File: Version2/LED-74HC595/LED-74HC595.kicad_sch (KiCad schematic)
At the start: 5 parts, among them J1 Conn_01x08_Pin, J2 Conn_01x08_Pin, J3 Conn_02x08_Odd_Even, U2 74HC595, U3 74HC595

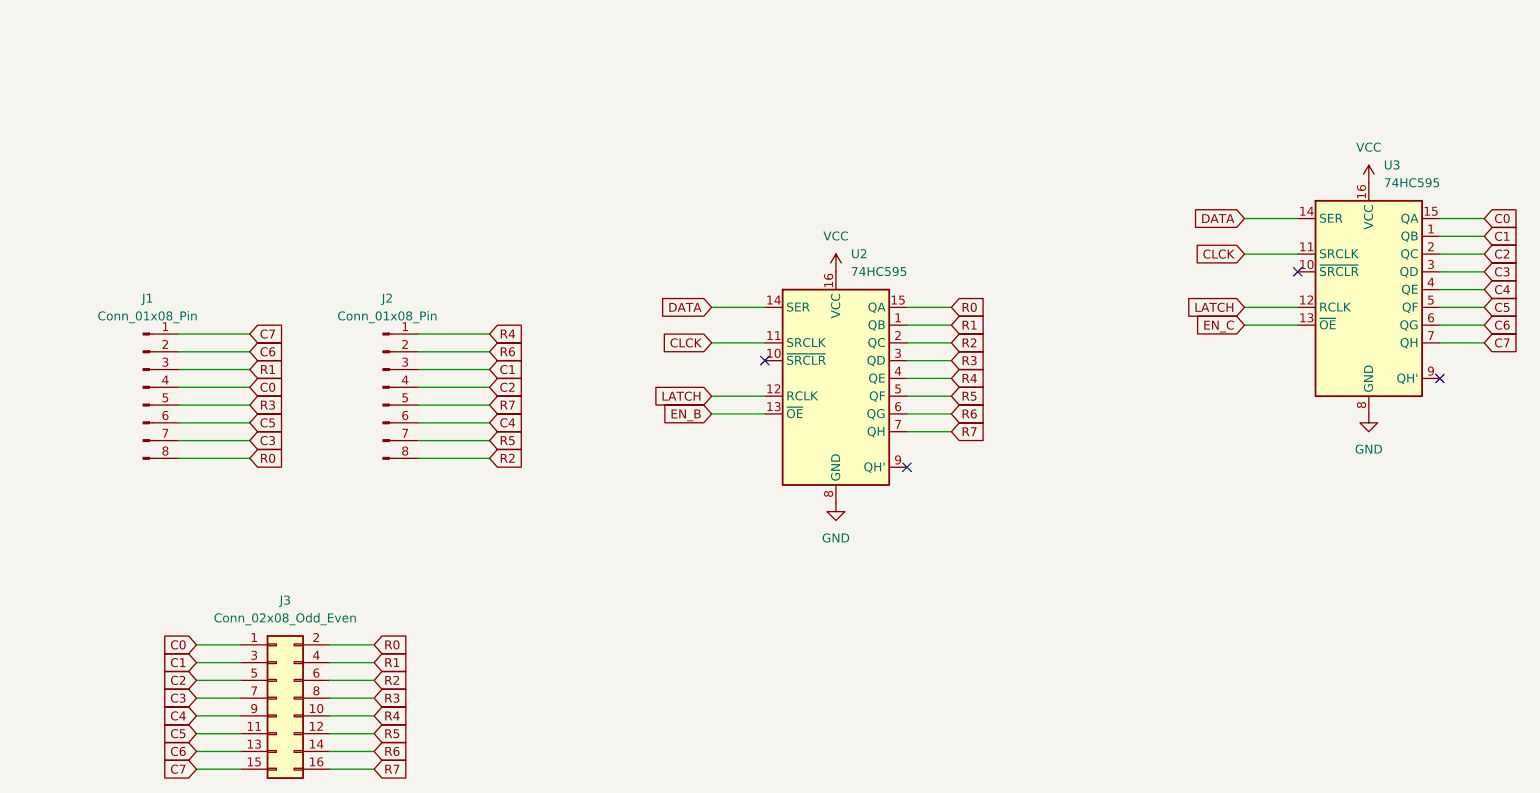
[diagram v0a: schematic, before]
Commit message: did some works.
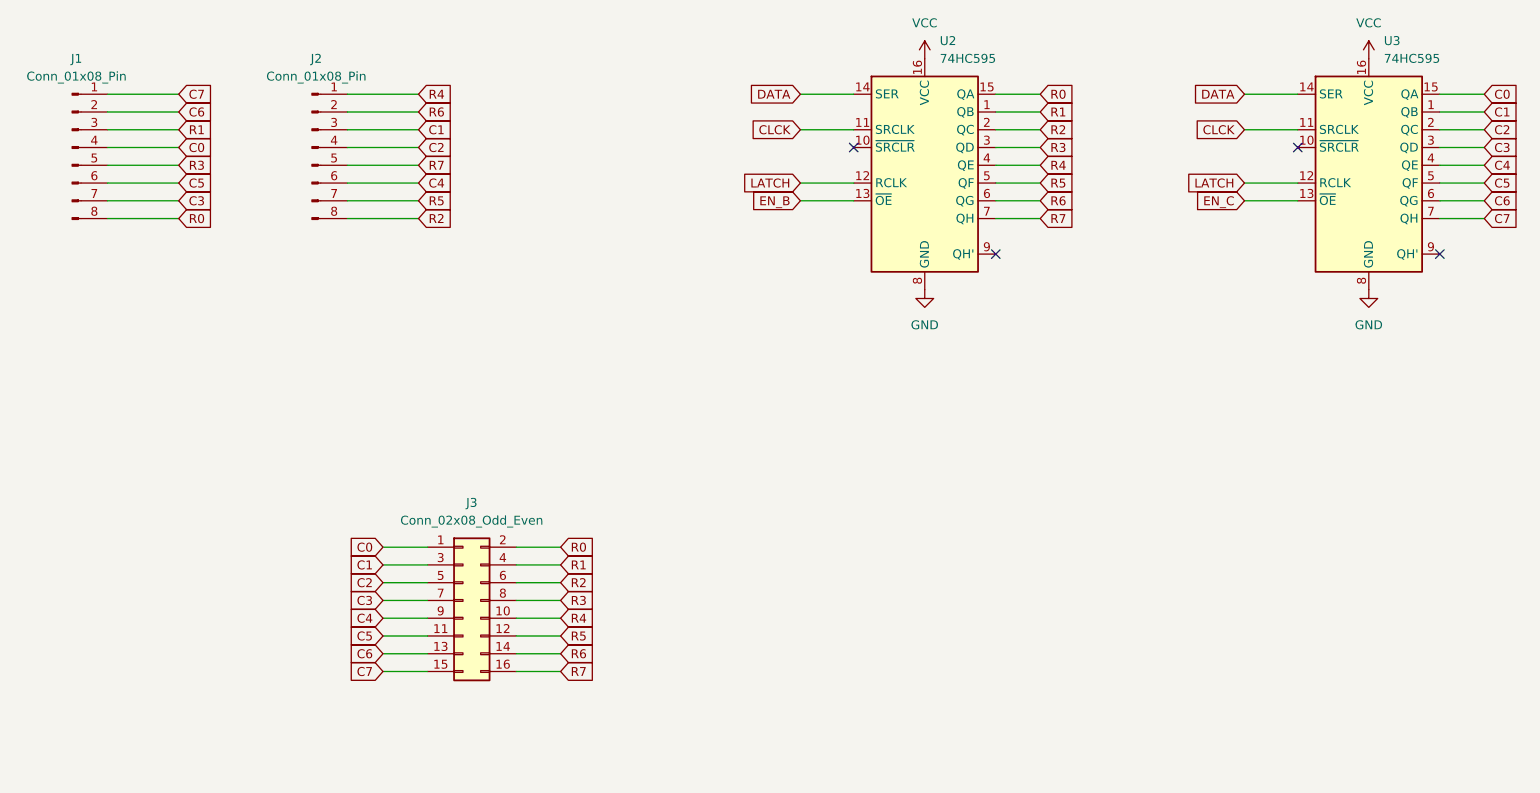
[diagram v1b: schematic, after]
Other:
- moved on the sheet: J1, J2, J3, U2, U3

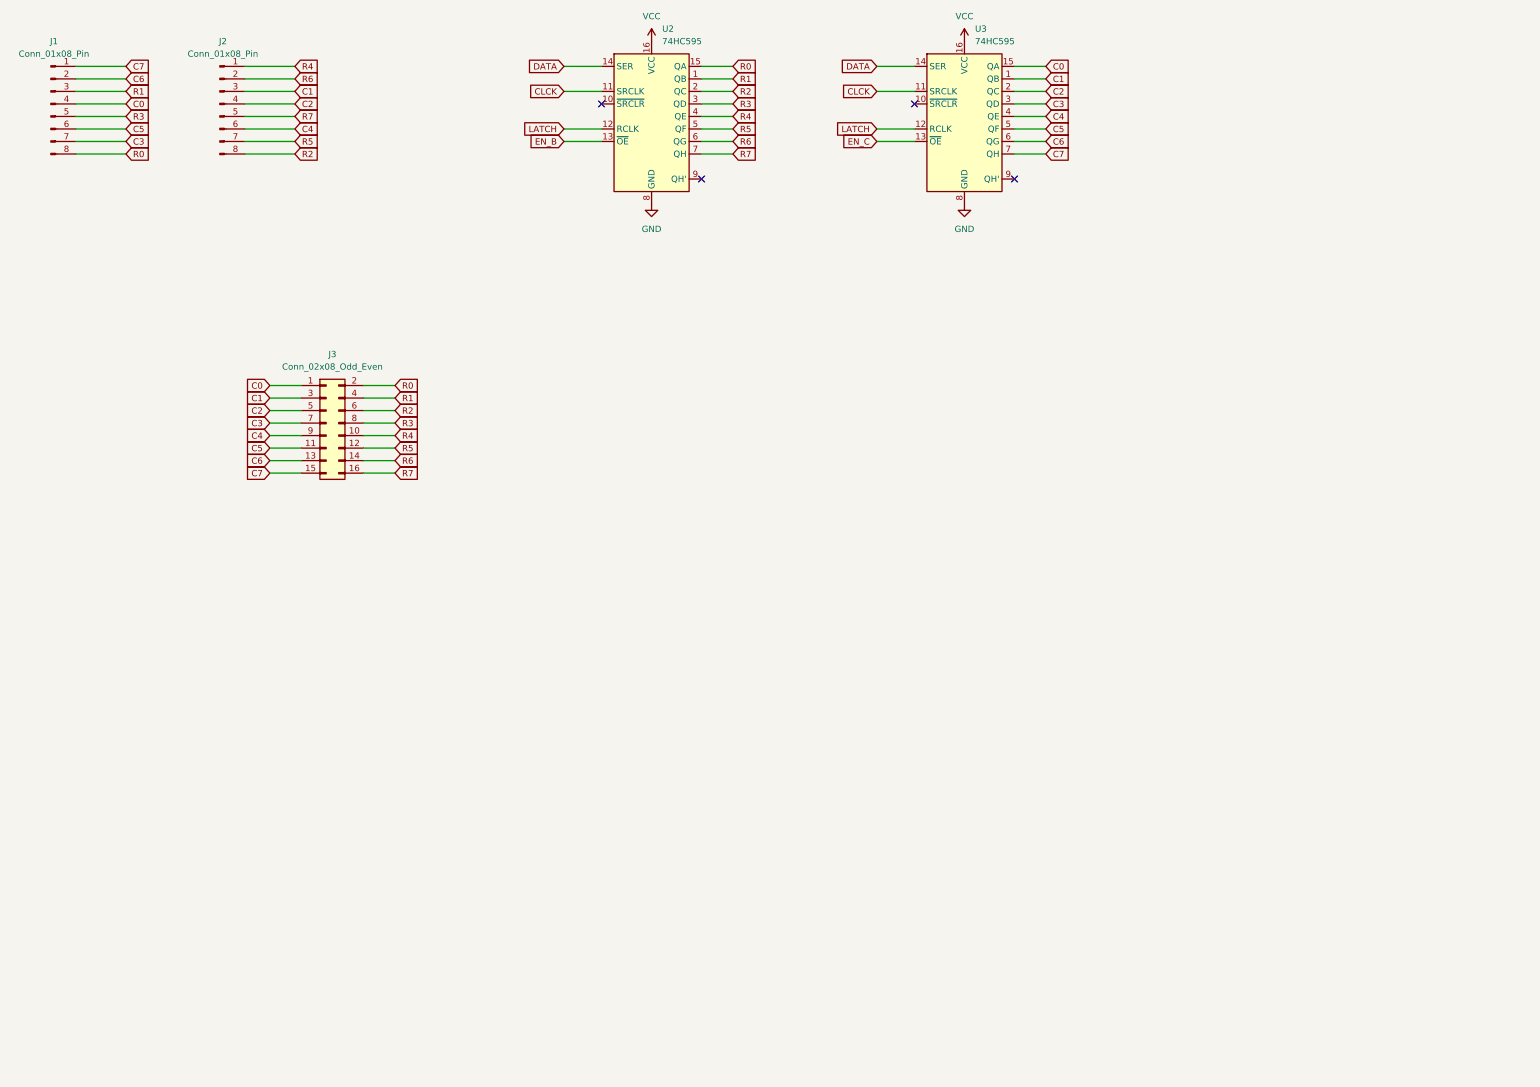
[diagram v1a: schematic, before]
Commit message: update.
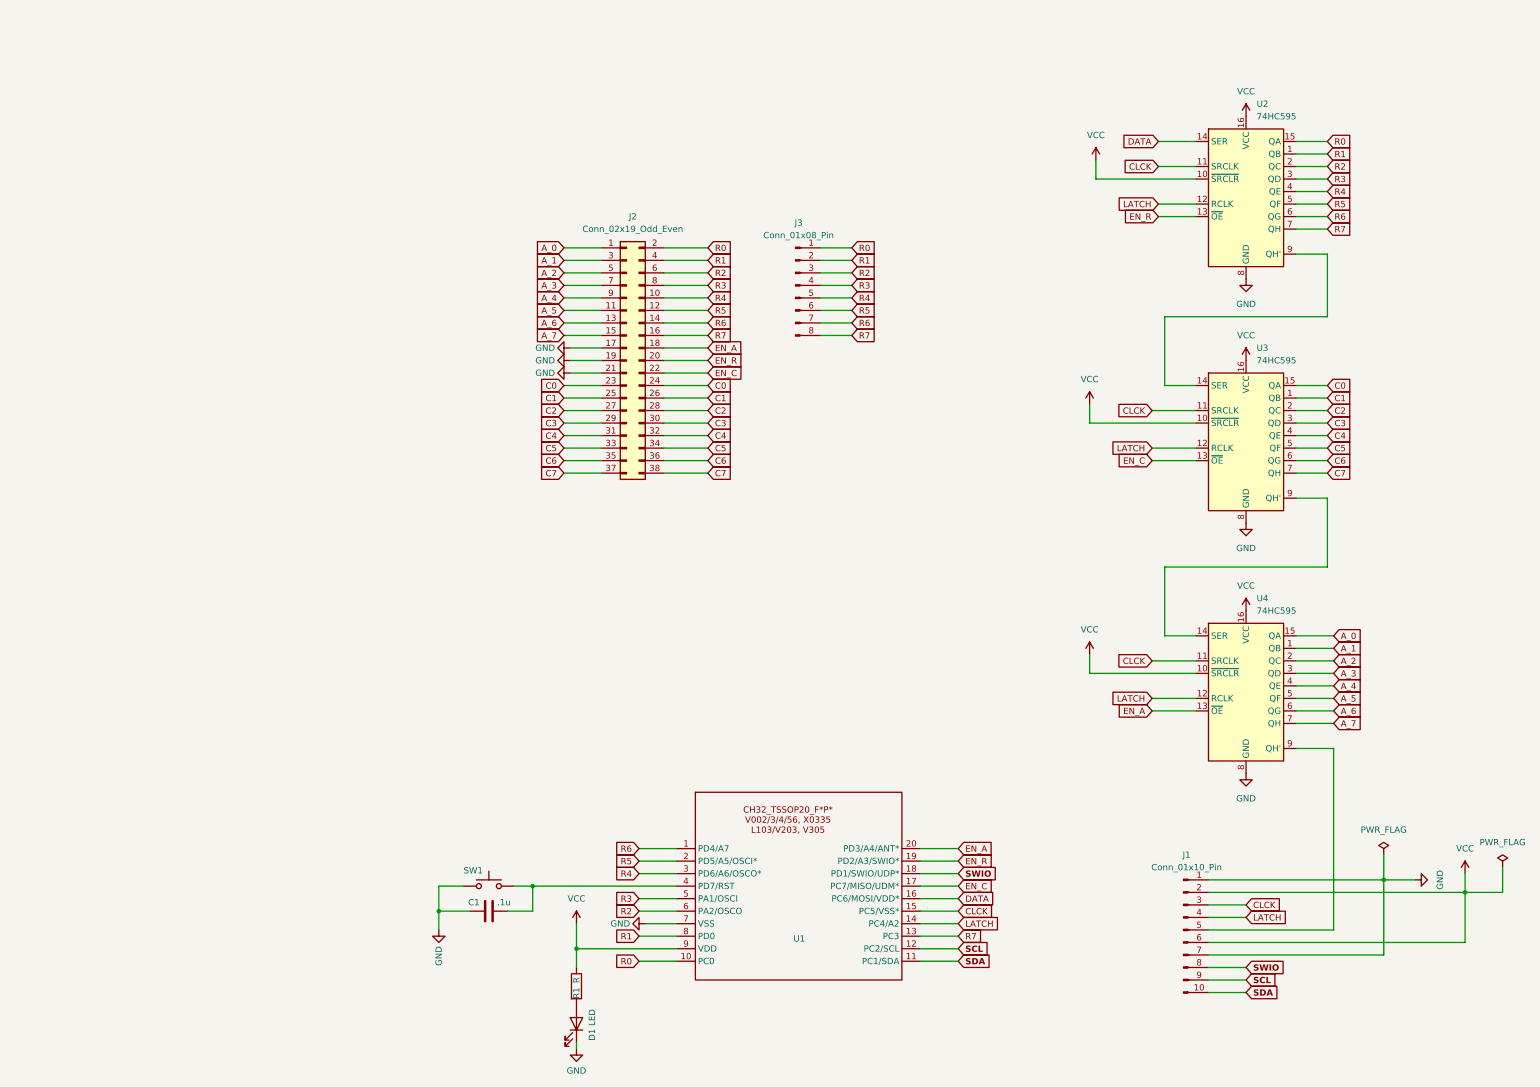
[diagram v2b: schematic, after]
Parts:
- removed J1: Conn_01x08_Pin, Connector_PinHeader_2.54mm:PinHeader_1x08_P2.54mm_Vertical, symbol Connector:Conn_01x08_Pin
- removed J3: Conn_02x08_Odd_Even, Connector_PinHeader_2.54mm:PinHeader_2x08_P2.54mm_Vertical, symbol Connector_Generic:Conn_02x08_Odd_Even
- added C1: .1u, Capacitor_SMD:C_0603_1608Metric, symbol Device:C
- added D1: LED, LED_SMD:LED_0603_1608Metric, symbol Device:LED
- added J1: Conn_01x10_Pin, Connector_PinHeader_2.54mm:PinHeader_1x10_P2.54mm_Vertical, symbol Connector:Conn_01x10_Pin
- added J2: Conn_02x19_Odd_Even, Connector_PinHeader_2.54mm:PinHeader_2x19_P2.54mm_Vertical, symbol Connector_Generic:Conn_02x19_Odd_Even
- added R1: R, Resistor_SMD:R_0603_1608Metric, symbol Device:R
- added SW1: SW_Push, Button_Switch_SMD:SW_SPST_PTS810, symbol Switch:SW_Push
- added U1: ~, Package_SO:TSSOP-20_4.4x6.5mm_P0.65mm, symbol IOT-Mess:CH32_TSSOP20_F*P*
- added U4: 74HC595, Package_SO:SOP-16_3.9x9.9mm_P1.27mm, symbol 74xx:74HC595
- renumbered J2 to J3
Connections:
- net C0: now also J2.23 (Pin_23), J2.24 (Pin_24)
- net C1: now also J2.25 (Pin_25), J2.26 (Pin_26); no longer J3.3 (Pin_3)
- net C2: now also J2.27 (Pin_27), J2.28 (Pin_28); no longer J3.4 (Pin_4)
- net C3: now also J2.29 (Pin_29), J2.30 (Pin_30)
- net C4: now also J2.31 (Pin_31), J2.32 (Pin_32); no longer J3.6 (Pin_6)
- net C5: now also J2.33 (Pin_33), J2.34 (Pin_34)
- net C6: now also J2.35 (Pin_35), J2.36 (Pin_36)
- net C7: now also J2.37 (Pin_37), J2.38 (Pin_38)
- net CLCK: now also J1.3 (Pin_3), U1.15 (PC5/VSS*), U4.11 (SRCLK)
- net DATA: now also U1.16 (PC6/MOSI/VDD*); no longer U3.14 (SER)
- net EN_C: now also J2.22 (Pin_22), U1.17 (PC7/MISO/UDM*)
- net GND: now also C1.2, D1.1 (K), J1.1 (Pin_1), J1.7 (Pin_7), J2.17 (Pin_17), J2.19 (Pin_19), J2.21 (Pin_21), SW1.1, U1.7 (VSS), U4.8 (GND)
- net LATCH: now also J1.4 (Pin_4), U1.14 (PC4/A2), U4.12 (RCLK)
- net R0: now also J3.1 (Pin_1), J2.2 (Pin_2), U1.10 (PC0)
- net R1: now also J3.2 (Pin_2), J2.4 (Pin_4), U1.8 (PD0)
- net R2: now also J3.3 (Pin_3), J2.6 (Pin_6), U1.6 (PA2/OSCO); no longer J3.8 (Pin_8)
- net R3: now also J3.4 (Pin_4), J2.8 (Pin_8), U1.5 (PA1/OSCI)
- net R4: now also J3.5 (Pin_5), J2.10 (Pin_10), U1.3 (PD6/A6/OSCO*); no longer J3.1 (Pin_1)
- net R5: now also J3.6 (Pin_6), J2.12 (Pin_12), U1.2 (PD5/A5/OSCI*); no longer J3.7 (Pin_7)
- net R6: now also J3.7 (Pin_7), J2.14 (Pin_14), U1.1 (PD4/A7); no longer J3.2 (Pin_2)
- net R7: now also J3.8 (Pin_8), J2.16 (Pin_16), U1.13 (PC3); no longer J3.5 (Pin_5)
- net VCC: now also U2.10 (~{SRCLR}), U3.10 (~{SRCLR}), J1.2 (Pin_2), J1.6 (Pin_6), R1.1, U1.9 (VDD), U4.10 (~{SRCLR}), U4.16 (VCC)
- net at U3.9 (QH'): now also U4.14 (SER)
- net at U2.9 (QH'): now also U3.14 (SER)
- net EN_B renamed EN_R
- net EN_R: now also J2.20 (Pin_20), U1.19 (PD2/A3/SWIO*)
- new net: J1.5 (Pin_5), U4.9 (QH')
- new net: C1.1, SW1.2, U1.4 (PD7/RST)
- new net: D1.2 (A), R1.2
- new net A_0: J2.1 (Pin_1), U4.15 (QA)
- new net A_1: J2.3 (Pin_3), U4.1 (QB)
- new net A_2: J2.5 (Pin_5), U4.2 (QC)
- new net A_3: J2.7 (Pin_7), U4.3 (QD)
- new net A_4: J2.9 (Pin_9), U4.4 (QE)
- new net A_5: J2.11 (Pin_11), U4.5 (QF)
- new net A_6: J2.13 (Pin_13), U4.6 (QG)
- new net A_7: J2.15 (Pin_15), U4.7 (QH)
- new net EN_A: J2.18 (Pin_18), U1.20 (PD3/A4/ANT*), U4.13 (~{OE})
- new net SCL: J1.9 (Pin_9), U1.12 (PC2/SCL)
- new net SDA: J1.10 (Pin_10), U1.11 (PC1/SDA)
- new net SWIO: J1.8 (Pin_8), U1.18 (PD1/SWIO/UDP*)
- no-connect marks 4 -> 0
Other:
- moved on the sheet: J3, U2, U3
